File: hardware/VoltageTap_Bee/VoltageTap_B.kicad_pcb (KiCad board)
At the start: 2 copper layers, 50 x 105 mm, 147 parts, among them J1 Conn_01x09_Socket, J101 HRLV, J102 Conn_01x18_Pin, J16 USB_B_Micro, Q6 2N7002, SW1 SW_Push, SW2 SW_Push, U10 MCP2542FDxMF, U12 FT230XS, U2 MCU-MSM0G3507SPM, U203 2PD2150-QX, U204 2PD2150-QX, U205 2PD2150-QX, U206 2PD2150-QX, U207 2PD2150-QX, U208 2PD2150-QX, U209 2PD2150-QX, U210 2PD2150-QX, U211 2PD2150-QX, U212 2PD2150-QX, U213 2PD2150-QX, U214 2PD2150-QX, U215 2PD2150-QX, U216 2PD2150-QX, U217 PBQ76952PFBT, U218 FCX495, U3 STISO620, U4 RAA211805, U5 STISO620

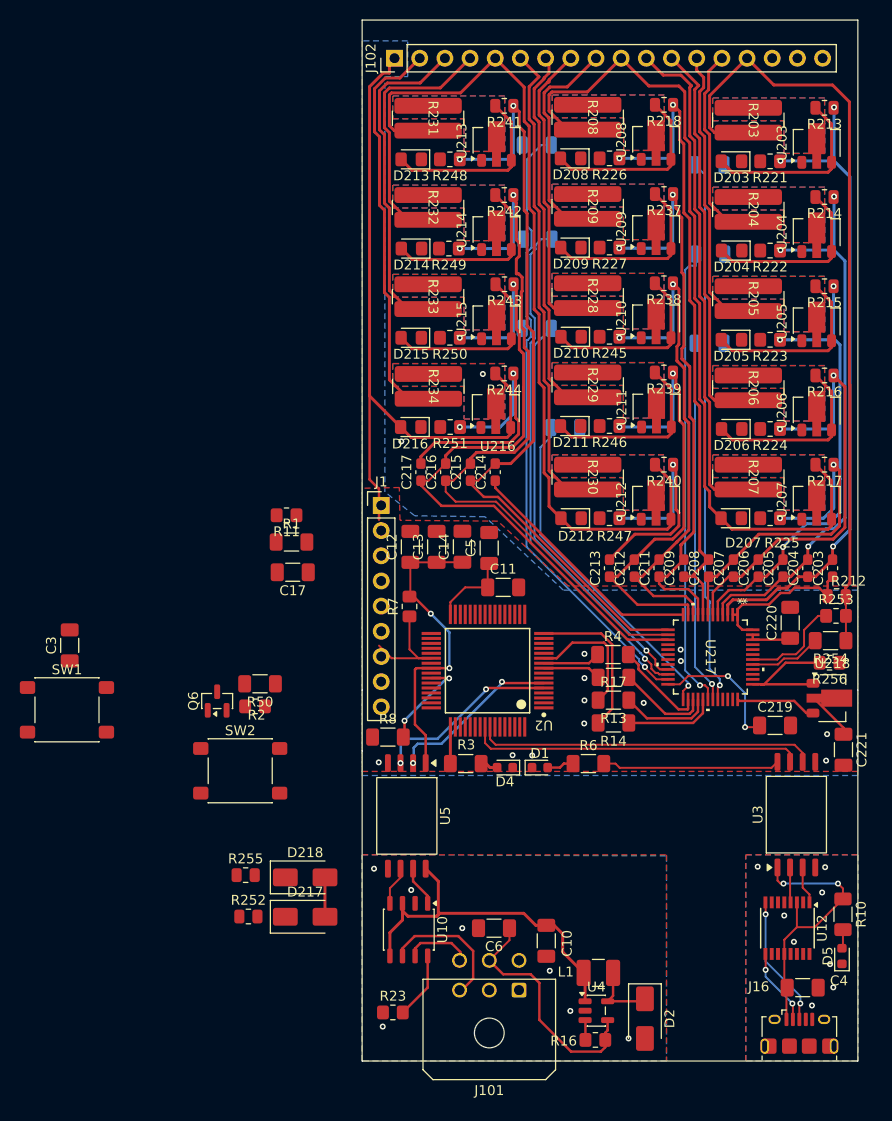
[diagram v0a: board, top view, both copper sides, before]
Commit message: This is a cry for help
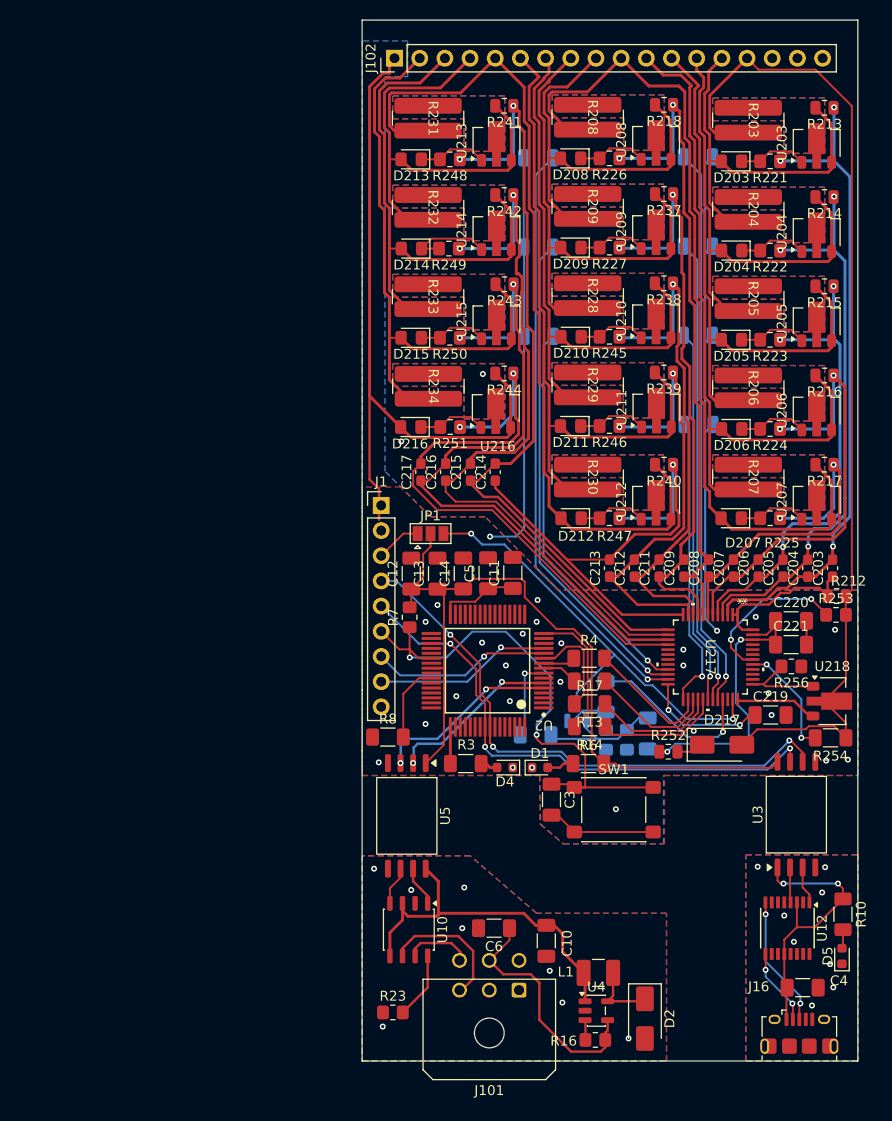
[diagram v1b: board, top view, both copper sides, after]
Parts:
- removed D218: ES1D, Diode_SMD:D_SMA
- removed R255: 100, Resistor_SMD:R_0805_2012Metric
- removed SW2: SW_Push, Button_Switch_SMD:SW_SPST_PTS645Sx43SMTR92
- added JP1: SolderJumper_3_Open, Jumper:SolderJumper-3_P1.3mm_Open_Pad1.0x1.5mm, F.Cu at (130.6, 83.7)
- C17, Q6, R1, R11, R2, R50: moved to B.Cu
- moved SW1 56.1 mm to (149.1, 111.5)
- moved C3 51.0 mm to (142.8, 110.5), turned to -90 degrees
- moved R252 45.5 mm to (154.6, 105.7)
- moved D217 45.5 mm to (160.0, 105.0)
- moved R11 41.1 mm to (150.4, 104.5), turned to 90 degrees
- moved C17 39.3 mm to (152.5, 103.9), turned to 90 degrees
- moved Q6 36.3 mm to (145.3, 101.7)
- moved R2 35.6 mm to (148.3, 104.5), turned to 90 degrees
- moved R50 34.9 mm to (148.3, 100.1), turned to -90 degrees
- moved R1 31.4 mm to (141.2, 104.0), turned to 180 degrees
- moved TH103 13.5 mm to (157.6, 72.7)
- moved C221 11.8 mm to (167.0, 94.9), turned to 0 degrees
- moved TH102 9.87 mm to (157.6, 54.7)
- moved R254 9.80 mm to (170.9, 104.3)
- moved TH104 8.30 mm to (157.6, 63.7)
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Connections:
- C221 pad 1: Net-(C221-Pad1) -> /BQ76952 1/BAT
- U218 pad 2: Net-(C221-Pad1) -> +BATT
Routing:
- net -BATT: track 71.4 -> 177.5 mm, vias 12 -> 27
- net onboard 3.3v src: track 0.00 -> 45.3 mm, vias 0 -> 2
- net RST_N: track 11.7 -> 53.6 mm, vias 0 -> 2
- net Net-(U217-VC0): track 27.9 -> 62.8 mm
- net VDD: track 49.2 -> 82.0 mm, vias 2 -> 0
- net /BQ76952 1/BAT: track 4.90 -> 29.4 mm, vias 0 -> 2
- net PA11_UART0-RX_XDS: track 34.2 -> 56.9 mm, vias 0 -> 3
- net PA10_UART0-TX_XDS: track 33.7 -> 54.5 mm, vias 0 -> 3
- net +BATT: track 83.4 -> 103.9 mm
- net PA19_SWDIO: track 0.00 -> 18.1 mm, vias 0 -> 1
- net PA20_SWCLK: track 0.00 -> 17.9 mm, vias 0 -> 1
- net /BQ76952 1/RST_SHUT: track 0.00 -> 17.6 mm, vias 0 -> 1
- net Net-(Q6-G): track 0.00 -> 13.0 mm
- net /BQ76952 1/DCHG: track 36.7 -> 47.4 mm
- net /BQ76952 1/DFETOFF: track 47.1 -> 37.9 mm
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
